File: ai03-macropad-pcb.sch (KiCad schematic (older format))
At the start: 76 parts, among them J1 Conn_01x06, SW1 SW_Push, U1 ATmega32U4-MU, Y1 16Mhz

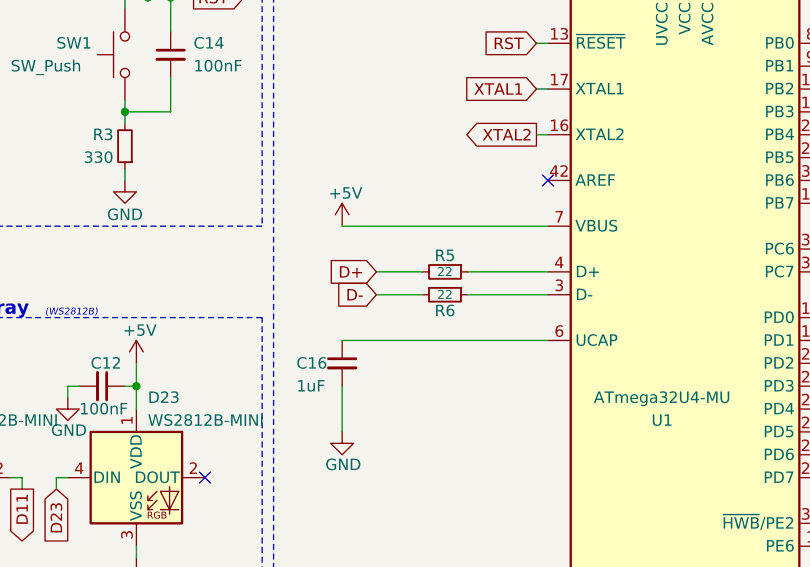
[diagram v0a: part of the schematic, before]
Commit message: RevA DRC check
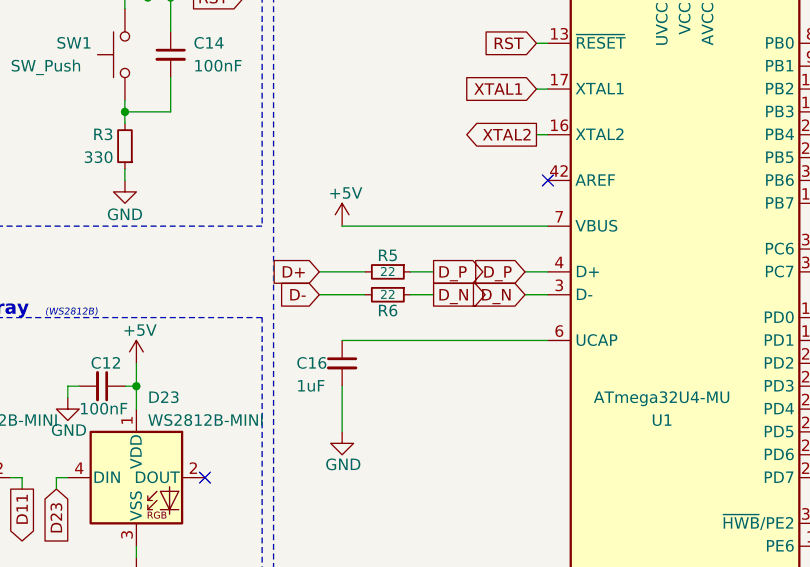
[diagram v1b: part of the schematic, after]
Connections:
- net D_N: now reaches R6.1, U1.3 (D-)
- net D_P: now reaches R5.1, U1.4 (D+)
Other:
- moved on the sheet: R5, R6
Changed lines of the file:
@@
 L Device:R_Small R6
 U 1 1 6073035A
-P 8450 3800
-F 0 "R6" V 8550 3800 50  0000 C BNN
-F 1 "22" V 8450 3800 39  0000 C CNN
-F 2 "Resistor_SMD:R_0603_1608Metric" H 8450 3800 50  0001 C CNN
-F 3 "~" H 8450 3800 50  0001 C CNN
-	1    8450 3800
+P 8200 3800
+F 0 "R6" V 8300 3800 50  0000 C BNN
+F 1 "22" V 8200 3800 39  0000 C CNN
+F 2 "Resistor_SMD:R_0603_1608Metric" H 8200 3800 50  0001 C CNN
+F 3 "~" H 8200 3800 50  0001 C CNN
+	1    8200 3800
 	0    1    1    0
 $EndComp
@@
 L Device:R_Small R5
 U 1 1 6072EE07
-P 8450 3700
-F 0 "R5" V 8350 3700 50  0000 C TNN
-F 1 "22" V 8450 3700 39  0000 C CNN
-F 2 "Resistor_SMD:R_0603_1608Metric" H 8450 3700 50  0001 C CNN
-F 3 "~" H 8450 3700 50  0001 C CNN
-	1    8450 3700
+P 8200 3700
+F 0 "R5" V 8100 3700 50  0000 C TNN
+F 1 "22" V 8200 3700 39  0000 C CNN
+F 2 "Resistor_SMD:R_0603_1608Metric" H 8200 3700 50  0001 C CNN
+F 3 "~" H 8200 3700 50  0001 C CNN
+	1    8200 3700
 	0    1    1    0
 $EndComp
@@
 	5250 7200 5250 7250
 Wire Wire Line
-	8150 3800 8350 3800
-Wire Wire Line
-	8150 3700 8350 3700
-Wire Wire Line
-	8900 3800 8550 3800
-Wire Wire Line
-	8550 3700 8900 3700
-Text GLabel 8150 3800 0    50   Input ~ 0
+	7900 3800 8100 3800
+Wire Wire Line
+	7900 3700 8100 3700
+Text GLabel 7900 3800 0    50   Input ~ 0
 D-
-Text GLabel 8150 3700 0    50   Input ~ 0
+Text GLabel 7900 3700 0    50   Input ~ 0
 D+
 $Comp
@@
 NoConn ~ 10100 2700
 NoConn ~ 10100 5600
+Wire Wire Line
+	8300 3700 8400 3700
+Wire Wire Line
+	8300 3800 8400 3800
+Wire Wire Line
+	8900 3700 8800 3700
+Wire Wire Line
+	8900 3800 8800 3800
+Text GLabel 8800 3800 0    50   Input ~ 0
+D_N
+Text GLabel 8400 3800 2    50   Output ~ 0
+D_N
+Text GLabel 8400 3700 2    50   Output ~ 0
+D_P
+Text GLabel 8800 3700 0    50   Input ~ 0
+D_P
 $EndSCHEMATC
